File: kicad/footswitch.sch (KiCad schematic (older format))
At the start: 37 parts

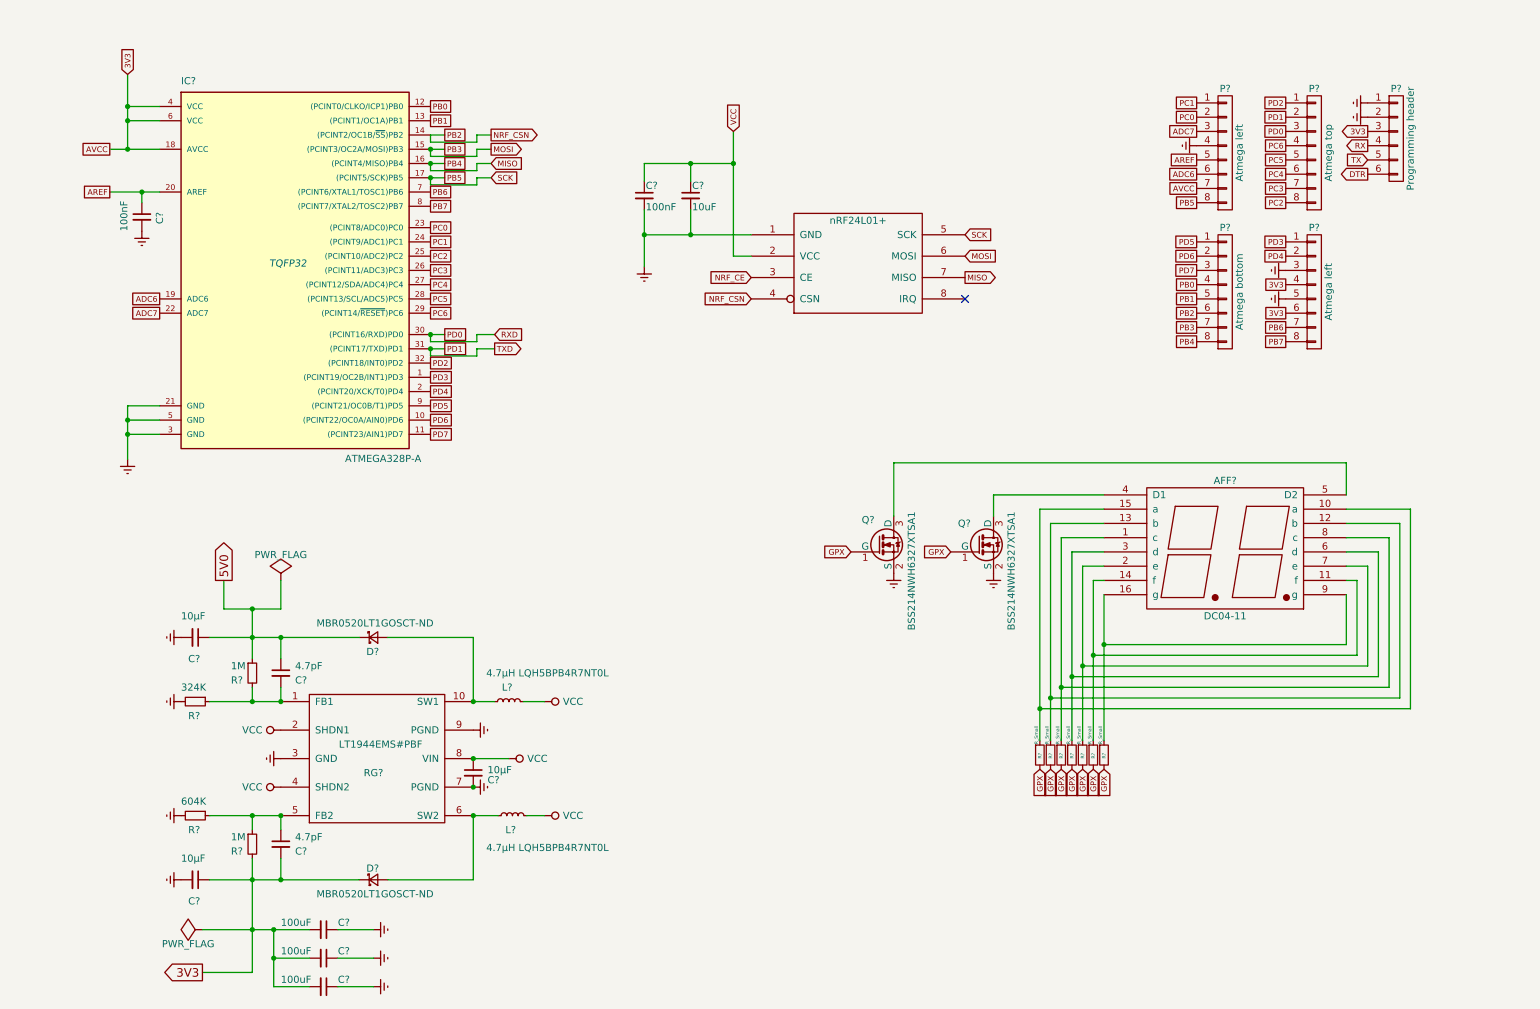
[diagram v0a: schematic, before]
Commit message: Continue schematic
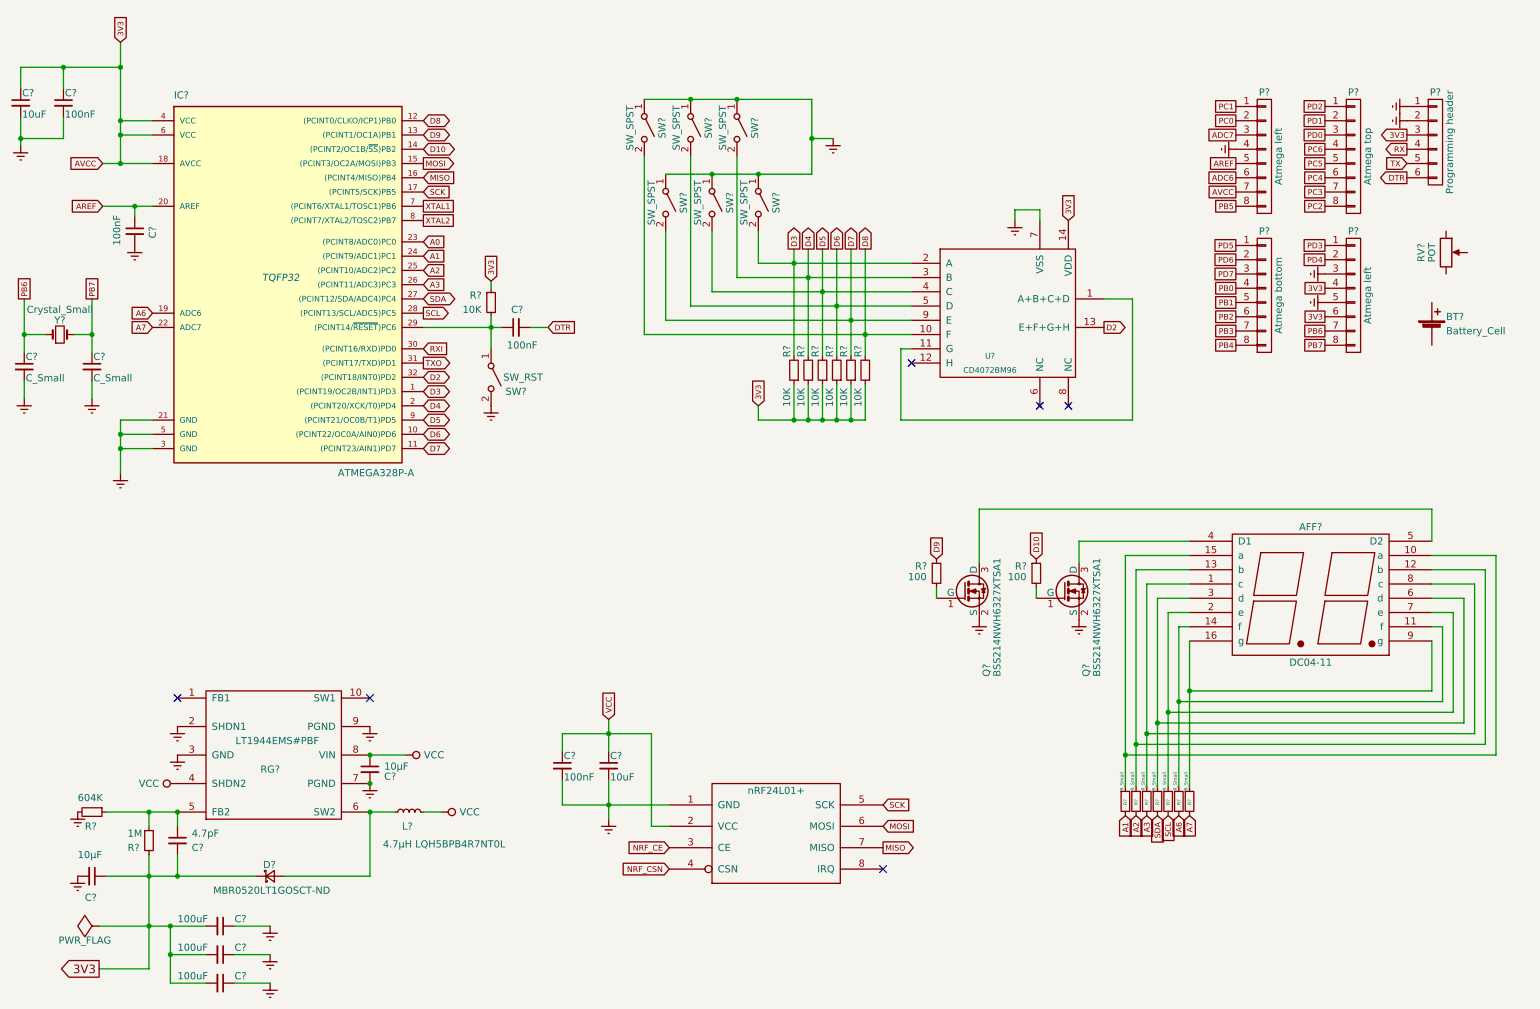
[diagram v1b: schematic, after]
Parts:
- removed C?: 4.7pF, Capacitors_SMD:C_0805_HandSoldering, symbol C_Small
- removed C?: 10µF, Capacitors_SMD:C_0805_HandSoldering, symbol C_Small
- removed D?: MBR0520LT1GOSCT-ND, Diodes_SMD:SOD-123, symbol D_Schottky_Small
- removed L?: 4.7µH LQH5BPB4R7NT0L, symbol L_Small
- removed R?: 1M, Resistors_SMD:R_0805_HandSoldering, symbol R_Small
- removed R?: 324K, Resistors_SMD:R_0805_HandSoldering, symbol R_Small
- added BT?: Battery_Cell, symbol Battery_Cell
- added C? (x2): C_Small, symbol C_Small
- added C? (x2): 100nF, symbol C_Small
- added C?: 10uF, symbol C_Small
- added R? (x2): 100, symbol R_Small
- added R?: 10K, symbol R_Small
- added R? (x6): 10K, Resistors_SMD:R_0805_HandSoldering, symbol R_Small
- added RV?: POT, symbol POT
- added SW? (x6): SW_SPST, symbol SW_SPST
- added SW?: SW_RST, symbol SW_SPST
- added U?: CD4072BM96, symbol CD4072BM96
- added Y?: Crystal_Small, symbol Crystal_Small
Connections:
- net 3V3: now also C?.1, C?.1, R?.1, R?.1, R?.1, R?.1, R?.1, R?.1, R?.1, U?.14 (VDD)
- net ADC6: no longer IC?.19 (ADC6)
- net ADC7: no longer IC?.22 (ADC7)
- net DTR: now also C?.2
- net Earth: now also RG?.2 (SHDN1), C?.2, C?.2, C?.2, C?.2, SW?.1 (A), SW?.1 (A), SW?.1 (A), SW?.1 (A), SW?.1 (A), SW?.1 (A), SW?.2 (B), U?.7 (VSS)
- net MISO: no longer P?.8 (P8)
- net MOSI: no longer P?.7 (P7)
- net NRF_CSN: no longer IC?.14 ((PCINT2/OC1B/~SS~)PB2), P?.6 (P6)
- net PB0: no longer IC?.12 ((PCINT0/CLKO/ICP1)PB0)
- net PB1: no longer IC?.13 ((PCINT1/OC1A)PB1)
- net PB5: no longer IC?.17 ((PCINT5/SCK)PB5), U?.5 (SCK)
- net PB6: now also C?.1, Y?.1; no longer IC?.7 ((PCINT6/XTAL1/TOSC1)PB6)
- net PB7: now also C?.1, Y?.2; no longer IC?.8 ((PCINT7/XTAL2/TOSC2)PB7)
- net PC0: no longer IC?.23 ((PCINT8/ADC0)PC0)
- net PC1: no longer IC?.24 ((PCINT9/ADC1)PC1)
- net PC2: no longer IC?.25 ((PCINT10/ADC2)PC2)
- net PC3: no longer IC?.26 ((PCINT11/ADC3)PC3)
- net PC4: no longer IC?.27 ((PCINT12/SDA/ADC4)PC4)
- net PC5: no longer IC?.28 ((PCINT13/SCL/ADC5)PC5)
- net PC6: no longer IC?.29 ((PCINT14/~RESET~)PC6)
- net PD0: no longer IC?.30 ((PCINT16/RXD)PD0)
- net PD1: no longer IC?.31 ((PCINT17/TXD)PD1)
- net PD2: no longer IC?.32 ((PCINT18/INT0)PD2)
- net PD3: no longer IC?.1 ((PCINT19/OC2B/INT1)PD3)
- net PD4: no longer IC?.2 ((PCINT20/XCK/T0)PD4)
- net PD5: no longer IC?.9 ((PCINT21/OC0B/T1)PD5)
- net PD6: no longer IC?.10 ((PCINT22/OC0A/AIN0)PD6)
- net PD7: no longer IC?.11 ((PCINT23/AIN1)PD7)
- net VCC: no longer RG?.2 (SHDN1)
- removed net GPX: Q?.1 (G), Q?.1 (G), R?.2, R?.2, R?.2, R?.2, R?.2, R?.2, R?.2
- new net: C?.1, IC?.29 ((PCINT14/~RESET~)PC6), R?.2, SW?.1 (A)
- new net: Q?.1 (G), R?.2 (x2)
- new net: U?.1 (A+B+C+D), U?.11 (G)
- new net A0: IC?.23 ((PCINT8/ADC0)PC0)
- new net A1: IC?.24 ((PCINT9/ADC1)PC1), R?.2
- new net A2: IC?.25 ((PCINT10/ADC2)PC2), R?.2
- new net A3: IC?.26 ((PCINT11/ADC3)PC3), R?.2
- new net A6: IC?.19 (ADC6), R?.2
- new net A7: IC?.22 (ADC7), R?.2
- new net D10: IC?.14 ((PCINT2/OC1B/~SS~)PB2), R?.1
- new net D2: IC?.32 ((PCINT18/INT0)PD2), U?.13 (E+F+G+H)
- new net D3: IC?.1 ((PCINT19/OC2B/INT1)PD3), R?.2, SW?.2 (B), U?.2 (A)
- new net D4: IC?.2 ((PCINT20/XCK/T0)PD4), R?.2, SW?.2 (B), U?.3 (B)
- new net D5: IC?.9 ((PCINT21/OC0B/T1)PD5), R?.2, SW?.2 (B), U?.4 (C)
- new net D6: IC?.10 ((PCINT22/OC0A/AIN0)PD6), R?.2, SW?.2 (B), U?.5 (D)
- new net D7: IC?.11 ((PCINT23/AIN1)PD7), R?.2, SW?.2 (B), U?.9 (E)
- new net D8: IC?.12 ((PCINT0/CLKO/ICP1)PB0), R?.2, SW?.2 (B), U?.10 (F)
- new net D9: IC?.13 ((PCINT1/OC1A)PB1), R?.1
- new net PB2: P?.6 (P6)
- new net PB3: P?.7 (P7)
- new net PB4: P?.8 (P8)
- new net RXI: IC?.30 ((PCINT16/RXD)PD0)
- new net SCK: IC?.17 ((PCINT5/SCK)PB5), U?.5 (SCK)
- new net SCL: IC?.28 ((PCINT13/SCL/ADC5)PC5), R?.2
- new net SDA: IC?.27 ((PCINT12/SDA/ADC4)PC4), R?.2
- new net TXO: IC?.31 ((PCINT17/TXD)PD1)
- new net XTAL1: IC?.7 ((PCINT6/XTAL1/TOSC1)PB6)
- new net XTAL2: IC?.8 ((PCINT7/XTAL2/TOSC2)PB7)
- no-connect marks 1 -> 6
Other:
- moved on the sheet: AFF?, C?, D?, IC?, L?, P?, Q?, R?, RG?
